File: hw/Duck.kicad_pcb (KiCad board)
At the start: 2 copper layers, 35.5 x 20.8 mm, 38 parts, among them J1 Conn_01x06, J2 Conn_01x06, J3 USB_C_Receptacle_USB2.0_14P, Q1 MMBT3904, Q2 MMBT3904, U1 ESP32-S3-PICO-1, U2 SPX3819M5-L-3-3, U3 INMP441, U4 MAX17048G+T10, U5 CH343P

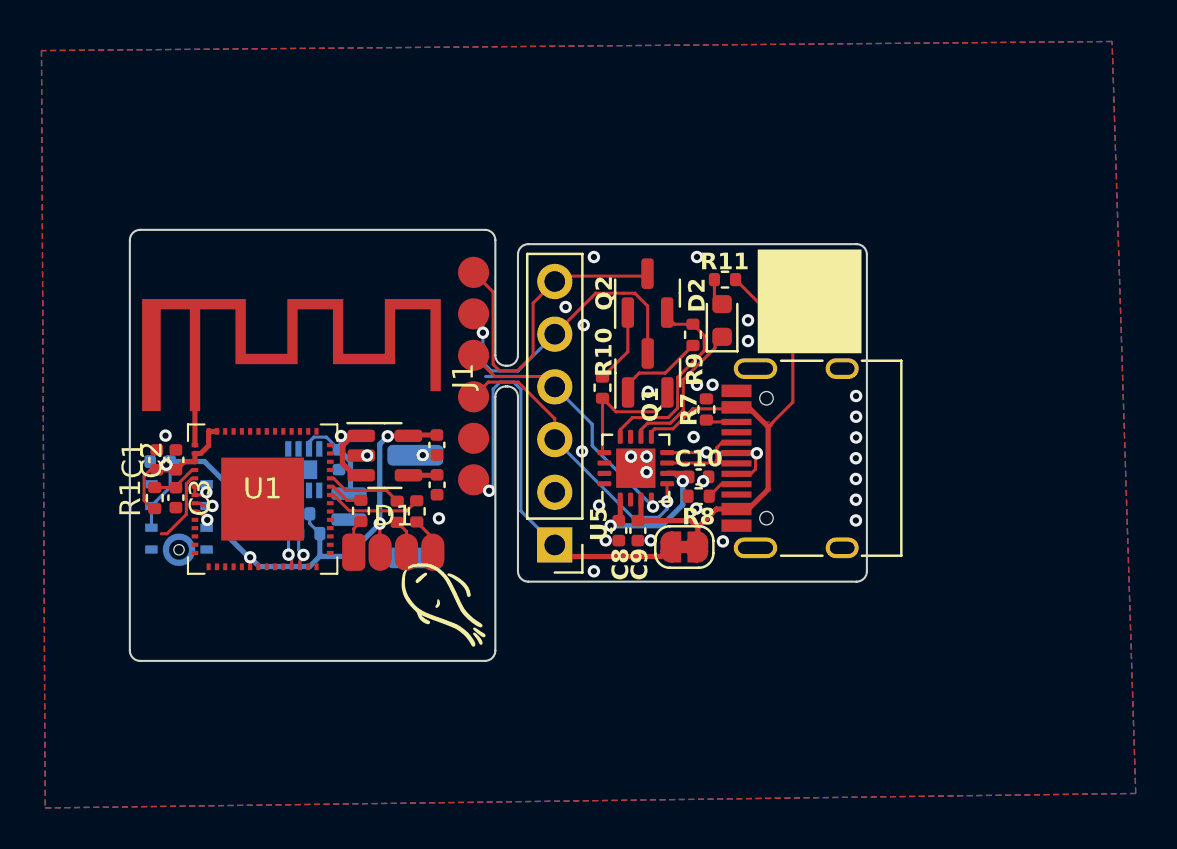
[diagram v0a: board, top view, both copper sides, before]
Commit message: hw: Complete revision
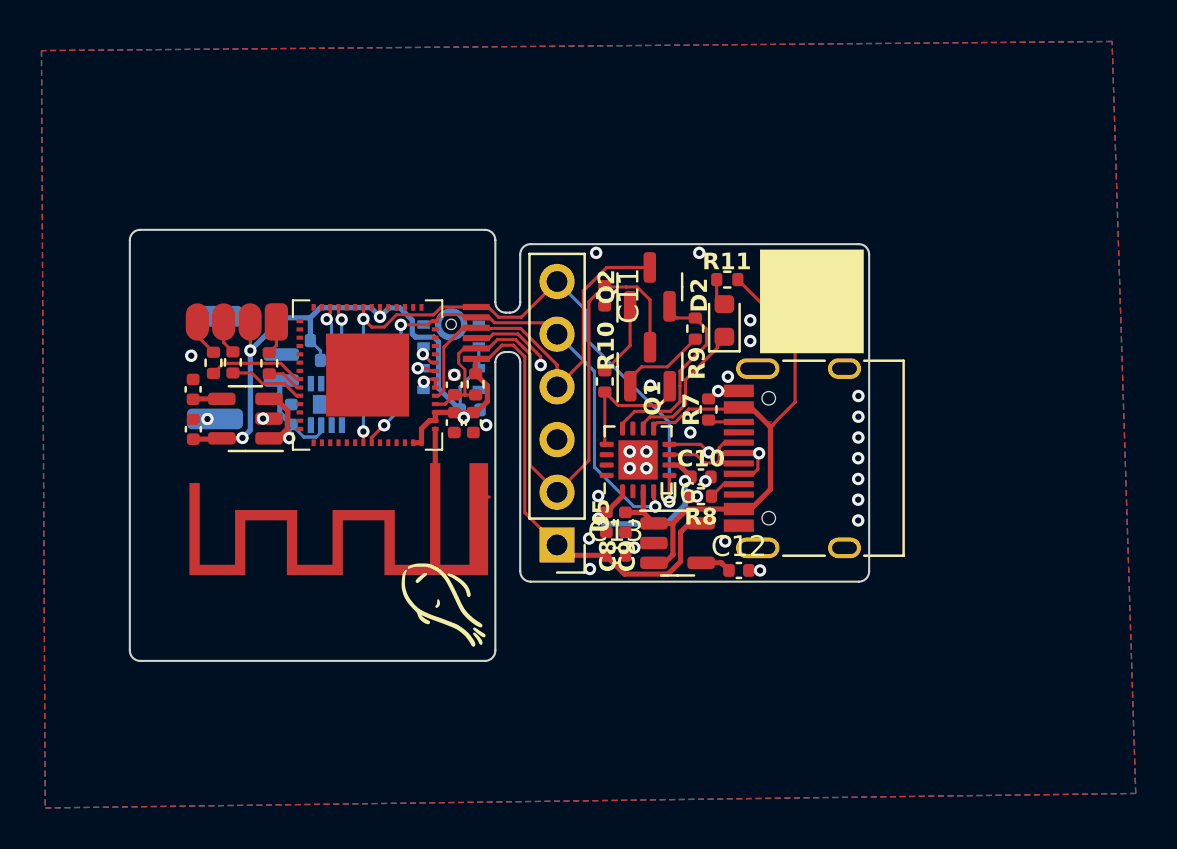
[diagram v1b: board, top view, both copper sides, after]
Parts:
- removed JP1: SolderJumper_2_Bridged, Jumper:SolderJumper-2_P1.3mm_Bridged_RoundedPad1.0x1.5mm
- added C11: 1u, Capacitor_SMD:C_0402_1005Metric, F.Cu at (79.4, 41.7)
- added C12: 10n, Capacitor_SMD:C_0402_1005Metric, F.Cu at (85.9, 54.9)
- added C13: 4.7u, Capacitor_SMD:C_0402_1005Metric, F.Cu at (79.9, 54.2)
- added U6: SPX3819M5-L-3-3, Package_TO_SOT_SMD:SOT-23-5, F.Cu at (82.9, 53.6)
- J1: footprint Duck_footprints:TestPoints_1x06_P2.0 -> Duck_footprints:TestPoints_FFC_1x06_P0.5
- moved R1 16.4 mm to (73.2, 45.9), turned to -90 degrees
- moved AE1 16.0 mm to (73.3, 49.7), turned to 0 degrees
- moved C1 15.4 mm to (73.1, 47.8), turned to -90 degrees
- moved U3 15.2 mm to (72.0, 44.6), turned to 90 degrees
- moved C6 15.1 mm to (72.9, 47.2), turned to 0 degrees
- moved C3 14.5 mm to (72.2, 46.0), turned to 90 degrees
- moved C2 13.5 mm to (72.2, 47.8), turned to -90 degrees
- moved D1 13.4 mm to (61.7, 42.9), turned to 180 degrees
- moved C4 12.6 mm to (59.6, 46.2), turned to 90 degrees
- moved R6 12.1 mm to (60.5, 44.9), turned to 90 degrees
- moved C5 11.8 mm to (59.6, 48.1), turned to 90 degrees
- moved R5 10.7 mm to (61.5, 44.9), turned to 90 degrees
- moved BT1 9.66 mm to (62.0, 45.1), turned to 90 degrees
- moved R2 9.32 mm to (65.7, 43.8), turned to 0 degrees
- moved R4 8.38 mm to (63.2, 44.9), turned to 90 degrees
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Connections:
- J1 pad 1: +BATT -> +3V3
- J1 pad 2: GND -> /ESP_EN
- J1 pad 3: /U0TXD -> GND
- J1 pad 4: /U0RXD -> /BOOT0
- J1 pad 5: /ESP_EN -> /U0RXD
- J1 pad 6: /BOOT0 -> /U0TXD
- J2 pad 1: +BATT -> +3V3
- J2 pad 2: GND -> /ESP_EN
- J2 pad 3: /U0TXD -> GND
- J2 pad 4: /U0RXD -> /BOOT0
- J2 pad 5: /ESP_EN -> /U0RXD
- J2 pad 6: /BOOT0 -> /U0TXD
- U1 pad 14: unconnected-(U1-GPIO9-Pad14) -> /U0RXD
- U1 pad 22: unconnected-(U1-GPIO16/XTAL_32K_N-Pad22) -> /U0TXD
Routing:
- net +3V3: track 36.0 -> 58.7 mm
- net +BATT: track 31.0 -> 9.27 mm, vias 2 -> 1
- net /U0TXD: track 14.3 -> 31.4 mm, vias 1 -> 3
- net /ESP_EN: track 17.2 -> 31.4 mm, vias 1 -> 0
- net /U0RXD: track 12.6 -> 25.6 mm, vias 1 -> 3
- net GND: track 2.13 -> 4.32 mm, vias 32 -> 33
- net VBUS: track 27.7 -> 29.8 mm
- net Net-(U6-BP): track 0.00 -> 1.50 mm
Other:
- board size 35.5 x 20.8 mm -> 35.6 x 20.8 mm
